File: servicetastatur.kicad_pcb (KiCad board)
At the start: 2 copper layers, 122 x 61 mm, 11 parts, among them J1 Conn_01x16_Socket, J2 Conn_01x06_Socket, U1 AT24CS16-SSHM, U2 TL7705A, U3 74HC165, U4 74HC00, U5 MC34063AP, U6 27C128, Y1 Crystal

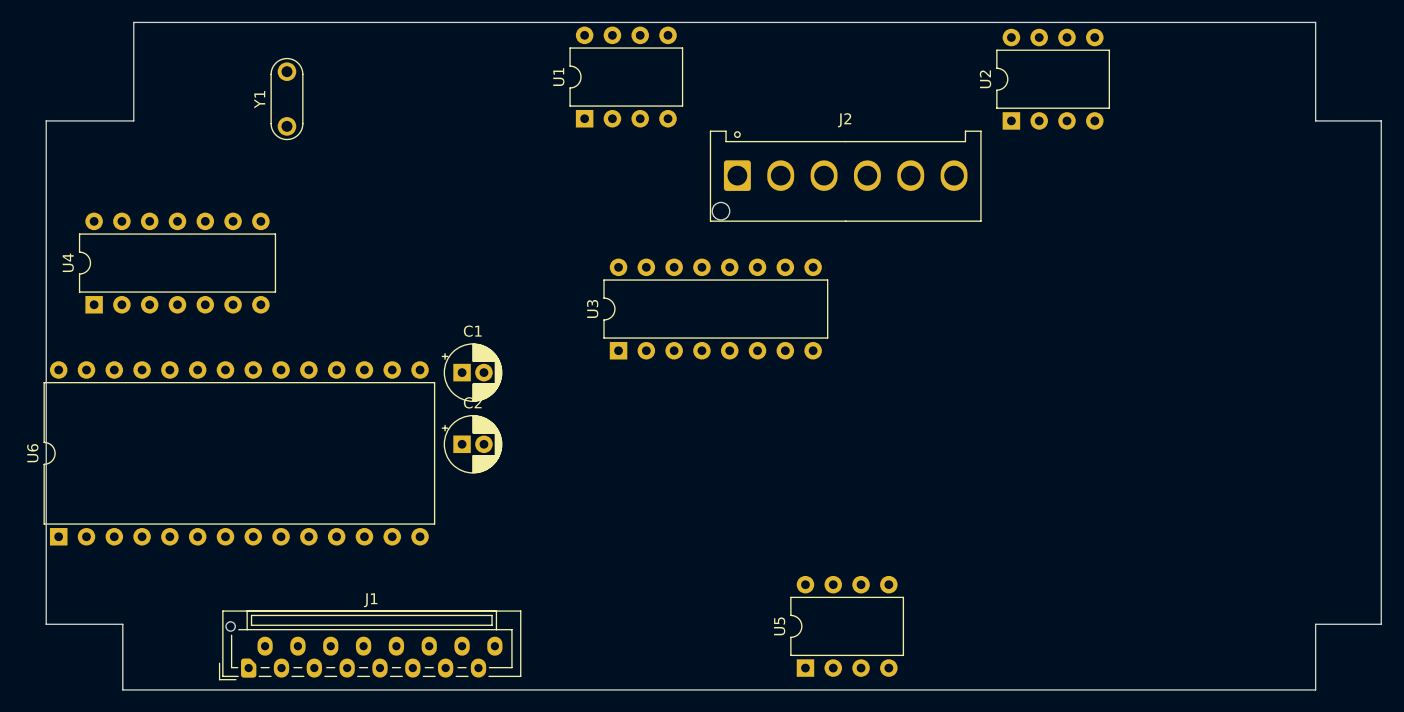
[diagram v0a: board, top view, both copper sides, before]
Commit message: war nochmal kleiner
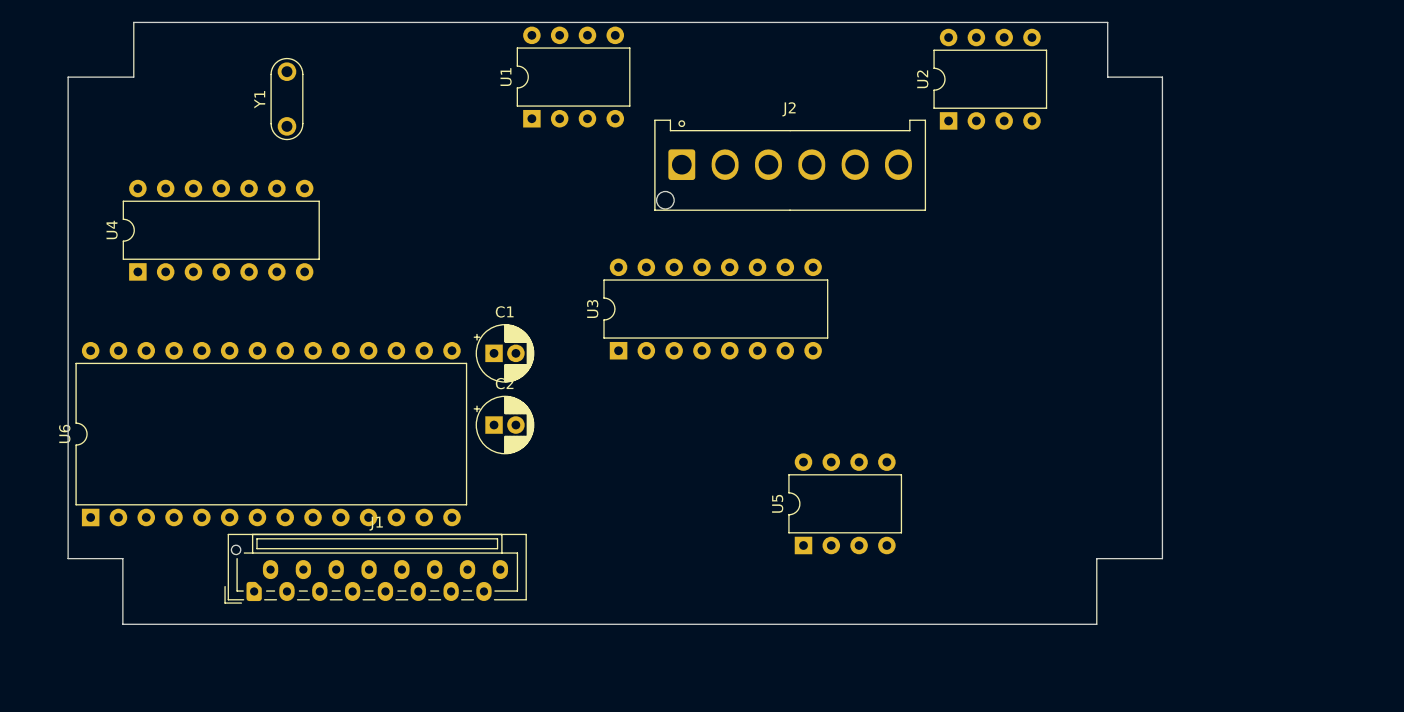
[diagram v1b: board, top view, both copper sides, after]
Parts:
- moved U5 11.2 mm to (147.2, 122.8)
- moved J1 7.02 mm to (97.0, 127.0)
- moved U2 5.74 mm to (160.5, 84.0)
- moved J2 5.18 mm to (136.1, 88.0)
- moved U4 5.00 mm to (86.4, 97.8)
- moved U1 4.82 mm to (122.4, 83.8)
- moved C1 3.41 mm to (118.9, 105.2)
- moved U6 3.41 mm to (82.1, 120.2)
- moved C2 3.41 mm to (118.9, 111.8)
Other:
- board size 122 x 61 mm -> 100 x 55 mm
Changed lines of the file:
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@@
   )
   (footprint "Package_DIP:DIP-8_W7.62mm" (layer "F.Cu")
-    (at 147.38 134 90)
+    (at 147.2 122.8 90)
     (descr "8-lead though-hole mounted DIP package, row spacing 7.62 mm (300 mils)")
     (tags "THT DIP DIL PDIP 2.54mm 7.62mm 300mil")
@@
   )
   (footprint "Connector_Hirose:Hirose_DF63-6P-3.96DSA_1x06_P3.96mm_Vertical" (layer "F.Cu")
-    (at 141.16 89)
+    (at 136.08 88)
     (descr "Hirose DF63 through hole, DF63-6P-3.96DSA, 6 Pins per row (https://www.hirose.com/product/en/products/DF63/), generated with kicad-footprint-generator")
     (tags "connector Hirose DF63 vertical")
@@
   )
   (footprint "Package_DIP:DIP-28_W15.24mm" (layer "F.Cu")
-    (at 79.14 122 90)
+    (at 82.06 120.24 90)
     (descr "28-lead though-hole mounted DIP package, row spacing 15.24 mm (600 mils)")
     (tags "THT DIP DIL PDIP 2.54mm 15.24mm 600mil")
@@
   )
   (footprint "Connector_JST:JST_ZE_B16B-ZESK-1D_1x16_P1.50mm_Vertical" (layer "F.Cu")
-    (at 96.5 134)
+    (at 97 127)
     (descr "JST ZE series connector, B16B-ZESK-1D, with boss (http://www.jst-mfg.com/product/pdf/eng/eZE.pdf), generated with kicad-footprint-generator")
     (tags "connector JST ZE side entry boss")
@@
   )
   (footprint "Capacitor_THT:CP_Radial_D5.0mm_P2.00mm" (layer "F.Cu")
-    (at 116 113.55)
+    (at 118.92 111.79)
     (descr "CP, Radial series, Radial, pin pitch=2.00mm, , diameter=5mm, Electrolytic Capacitor")
     (tags "CP Radial series Radial pin pitch 2.00mm  diameter 5mm Electrolytic Capacitor")
@@
   )
   (footprint "Package_DIP:DIP-8_W7.62mm" (layer "F.Cu")
-    (at 127.2 83.8 90)
+    (at 122.38 83.8 90)
     (descr "8-lead though-hole mounted DIP package, row spacing 7.62 mm (300 mils)")
     (tags "THT DIP DIL PDIP 2.54mm 7.62mm 300mil")
@@
   )
   (footprint "Package_DIP:DIP-14_W7.62mm" (layer "F.Cu")
-    (at 82.375 100.8 90)
+    (at 86.375 97.8 90)
     (descr "14-lead though-hole mounted DIP package, row spacing 7.62 mm (300 mils)")
     (tags "THT DIP DIL PDIP 2.54mm 7.62mm 300mil")
@@
   )
   (footprint "Capacitor_THT:CP_Radial_D5.0mm_P2.00mm" (layer "F.Cu")
-    (at 116 107)
+    (at 118.92 105.24)
     (descr "CP, Radial series, Radial, pin pitch=2.00mm, , diameter=5mm, Electrolytic Capacitor")
     (tags "CP Radial series Radial pin pitch 2.00mm  diameter 5mm Electrolytic Capacitor")
@@
   )
   (footprint "Package_DIP:DIP-8_W7.62mm" (layer "F.Cu")
-    (at 166.2 84 90)
+    (at 160.46 84 90)
     (descr "8-lead though-hole mounted DIP package, row spacing 7.62 mm (300 mils)")
     (tags "THT DIP DIL PDIP 2.54mm 7.62mm 300mil")
@@
     )
   )
-  (gr_line (start 85 136) (end 194 136)
+  (gr_line (start 85 130) (end 174 130)
     (stroke (width 0.1) (type default)) (layer "Edge.Cuts"))
-  (gr_line (start 194 75) (end 86 75)
+  (gr_line (start 175 75) (end 86 75)
     (stroke (width 0.1) (type default)) (layer "Edge.Cuts"))
-  (gr_line (start 85 130) (end 85 136)
+  (gr_line (start 85 130) (end 85 124)
     (stroke (width 0.1) (type default)) (layer "Edge.Cuts"))
-  (gr_line (start 78 84) (end 78 130)
+  (gr_line (start 80 80) (end 80 124)
     (stroke (width 0.1) (type default)) (layer "Edge.Cuts"))
-  (gr_line (start 78 130) (end 85 130)
+  (gr_line (start 80 124) (end 85 124)
     (stroke (width 0.1) (type default)) (layer "Edge.Cuts"))
-  (gr_line (start 194 136) (end 194 130)
+  (gr_line (start 174 130) (end 174 124)
     (stroke (width 0.1) (type default)) (layer "Edge.Cuts"))
-  (gr_line (start 194 130) (end 200 130)
+  (gr_line (start 174 124) (end 180 124)
     (stroke (width 0.1) (type default)) (layer "Edge.Cuts"))
-  (gr_line (start 194 84) (end 194 75)
+  (gr_line (start 175 80) (end 175 75)
     (stroke (width 0.1) (type default)) (layer "Edge.Cuts"))
-  (gr_line (start 86 84) (end 78 84)
+  (gr_line (start 86 80) (end 80 80)
     (stroke (width 0.1) (type default)) (layer "Edge.Cuts"))
-  (gr_line (start 200 84) (end 194 84)
+  (gr_line (start 180 80) (end 175 80)
     (stroke (width 0.1) (type default)) (layer "Edge.Cuts"))
-  (gr_line (start 86 75) (end 86 84)
+  (gr_line (start 86 75) (end 86 80)
     (stroke (width 0.1) (type default)) (layer "Edge.Cuts"))
-  (gr_line (start 200 130) (end 200 84)
+  (gr_line (start 180 124) (end 180 80)
     (stroke (width 0.1) (type default)) (layer "Edge.Cuts"))
 )
